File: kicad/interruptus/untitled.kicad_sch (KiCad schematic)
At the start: 16 parts, among them P2 USB_C_Plug_USB2.0, Q1 IRLML6402, U4 FT2232D, Y1 6Mhz

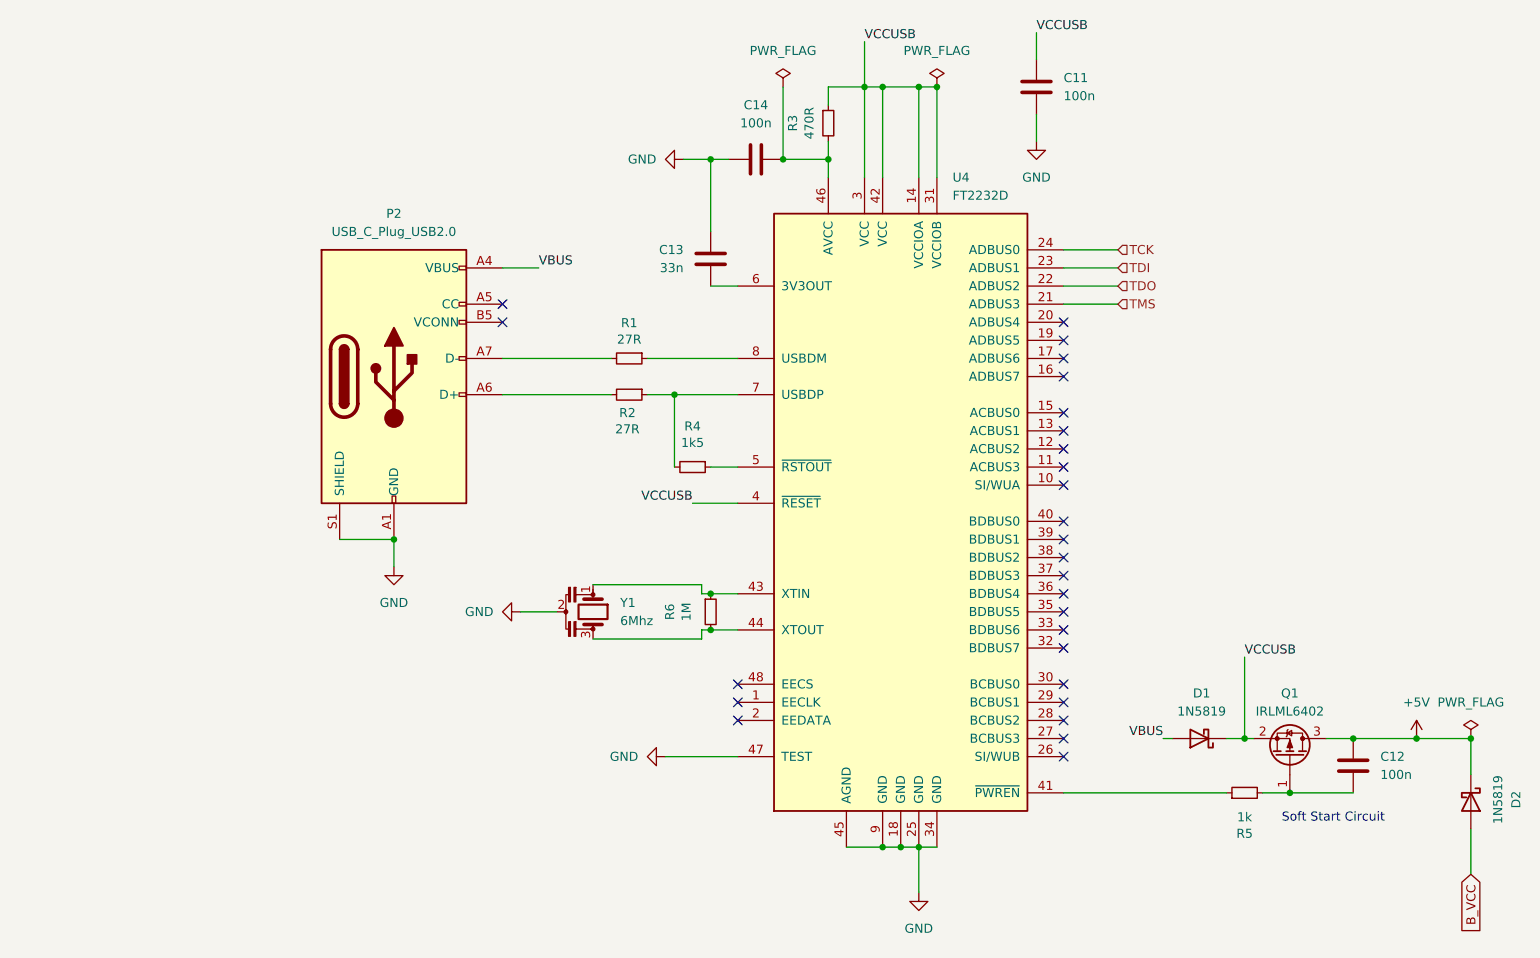
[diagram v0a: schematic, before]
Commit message: new usb connector, and other changes
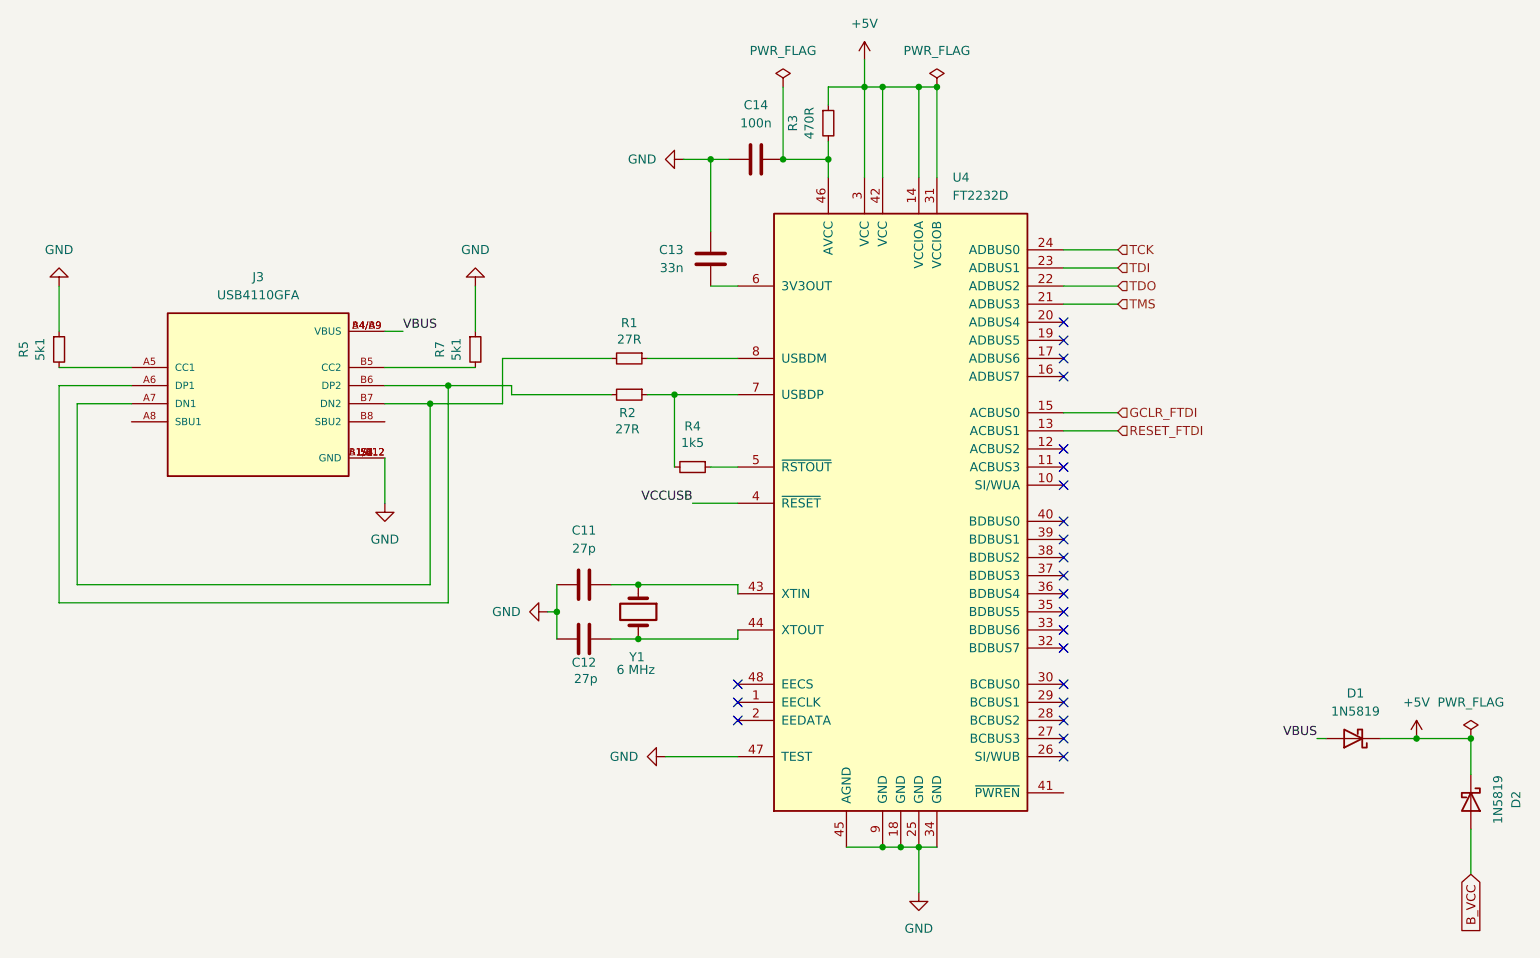
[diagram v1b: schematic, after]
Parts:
- removed P2: USB_C_Plug_USB2.0, Connector_USB:USB_C_Receptacle_G-Switch_GT-USB-7010ASV, symbol Connector:USB_C_Plug_USB2.0
- removed Q1: IRLML6402, Package_TO_SOT_SMD:SOT-23, symbol Transistor_FET:IRLML6402
- removed R6: 1M, Resistor_SMD:R_0201_0603Metric_Pad0.64x0.40mm_HandSolder, symbol Device:R_Small
- removed Y1: 6Mhz, Crystal:Resonator_Murata_CSTLSxxxX-3Pin_W5.5mm_H3.0mm, symbol Device:Resonator
- added J3: USB4110GFA, USB4110GFA:GCT_USB4110GFA, symbol USB4110GFA:USB4110GFA
- added R7: 5k1, Resistor_SMD:R_0201_0603Metric_Pad0.64x0.40mm_HandSolder, symbol Device:R_Small
- added Y1: 6 MHz, symbol Device:Crystal
- C11, C12: value 100n -> 27p
- R5: value 1k -> 5k1
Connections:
- net +5V: now also D1.1 (K), R3.1, U4.14 (VCCIOA), U4.3 (VCC), U4.31 (VCCIOB), U4.42 (VCC); no longer C12.1
- net GND: now also C11.1, C12.1, R5.1, J3.A1/B12 (GND), J3.B1/A12 (GND), J3.S1 (GND), J3.S2 (GND), J3.S3 (GND), J3.S4 (GND), R7.1; no longer C11.2
- net VBUS: now also J3.A4/B9 (VBUS), J3.B4/A9 (VBUS)
- net VCCUSB: no longer C11.1, D1.1 (K), R3.1, U4.14 (VCCIOA), U4.3 (VCC), U4.31 (VCCIOB), U4.42 (VCC)
- net at U4.43 (XTIN): now also C11.2, Y1.1
- net at U4.44 (XTOUT): now also C12.2, Y1.2
- net at U4.41 (~{PWREN}): no longer R5.1
- net at R5.2: now also J3.A5 (CC1); no longer C12.2
- net at R1.2: now also J3.A7 (DN1), J3.B7 (DN2)
- net at R2.2: now also J3.A6 (DP1), J3.B6 (DP2)
- net RESET_FTDI: now reaches U4.13 (ACBUS1)
- net GCLR_FTDI: now reaches U4.15 (ACBUS0)
- new net: J3.B5 (CC2), R7.2
- no-connect marks 27 -> 23
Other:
- note removed: "Soft Start Circuit"
- moved on the sheet: D1
